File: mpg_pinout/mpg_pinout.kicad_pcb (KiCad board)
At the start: 2 copper layers, 9 parts, among them J1 Conn_02x05_Odd_Even, J2 Conn_01x02_Pin, J3 Conn_01x02_Pin, J4 Conn_01x02_Pin, J5 Conn_01x02_Pin, J6 Conn_01x02_Pin, J7 Conn_01x02_Pin, J8 Conn_01x02_Pin

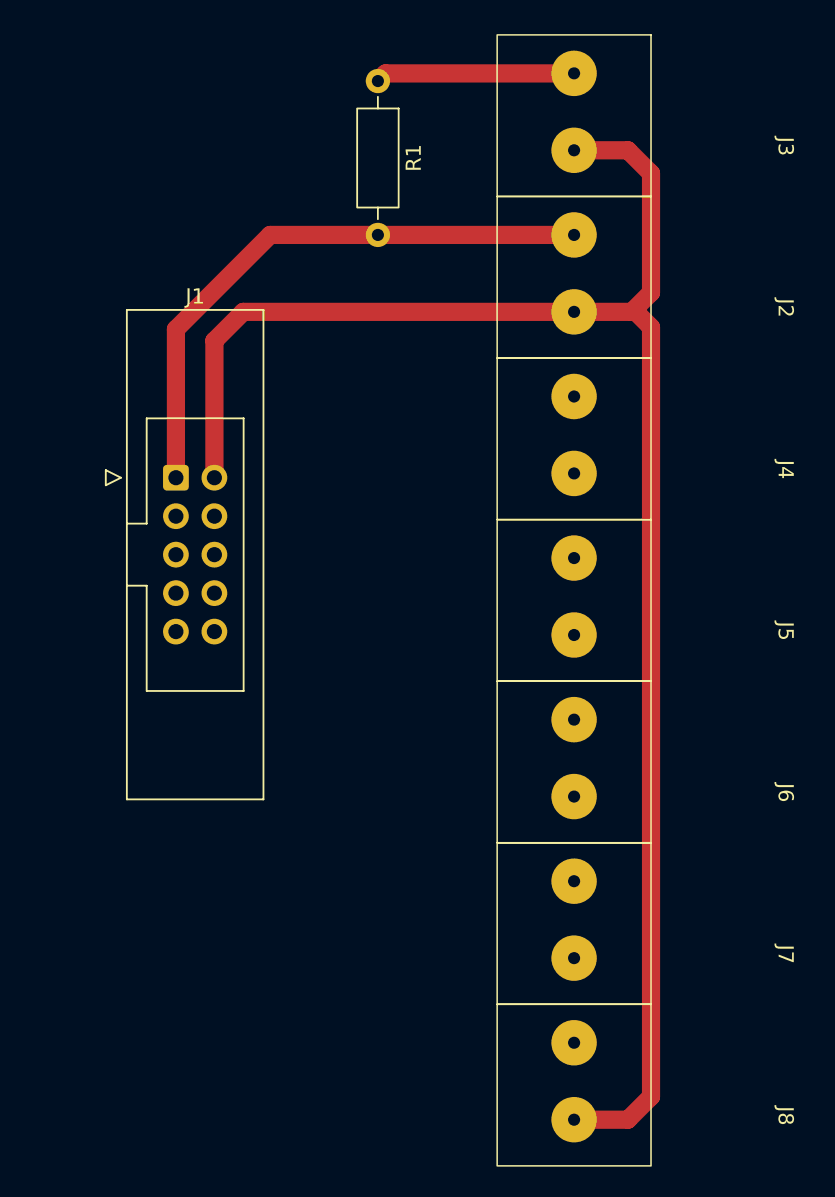
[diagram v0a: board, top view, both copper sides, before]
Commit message: third commit
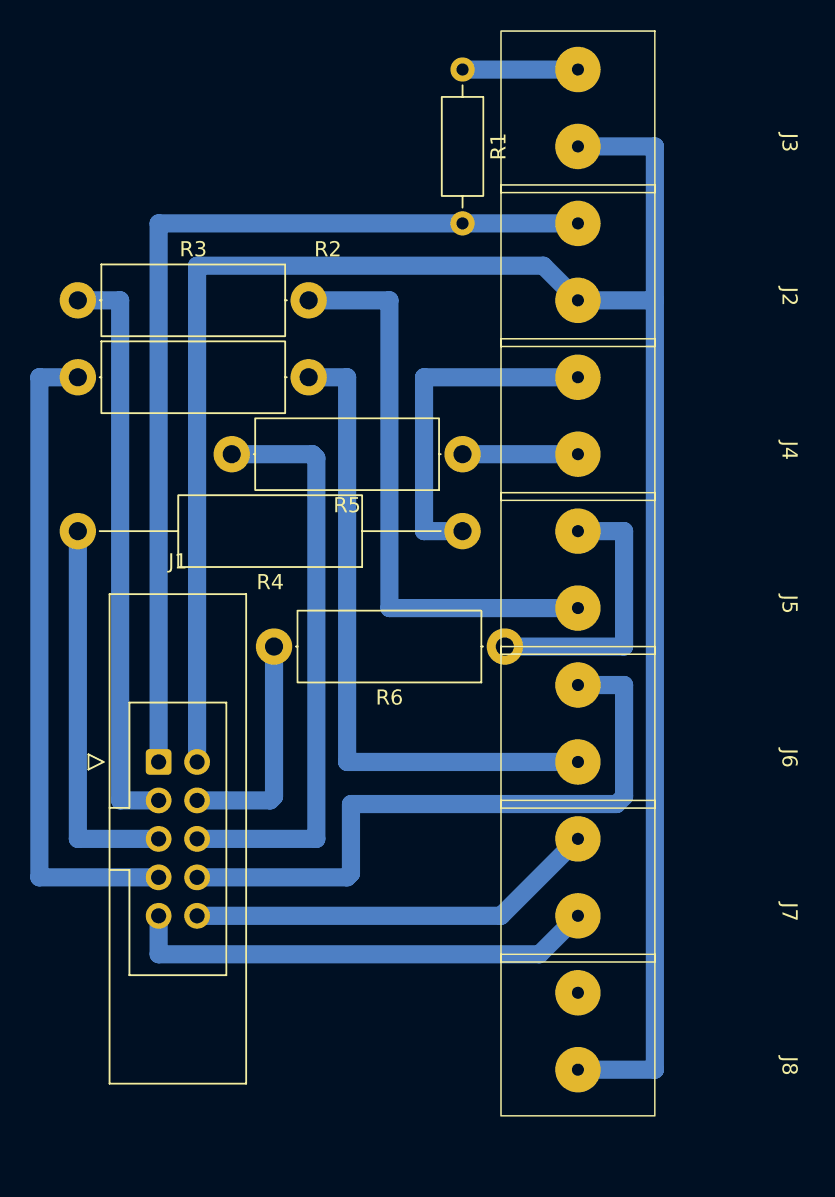
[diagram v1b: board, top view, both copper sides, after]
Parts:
- added R2: R, Resistor_THT:R_Axial_DIN0414_L11.9mm_D4.5mm_P15.24mm_Horizontal, F.Cu at (78.7, 61.0)
- added R3: R, Resistor_THT:R_Axial_DIN0414_L11.9mm_D4.5mm_P15.24mm_Horizontal, F.Cu at (78.7, 66.0)
- added R4: R, Resistor_THT:R_Axial_DIN0414_L11.9mm_D4.5mm_P25.40mm_Horizontal, F.Cu at (104.1, 76.2)
- added R5: R, Resistor_THT:R_Axial_DIN0414_L11.9mm_D4.5mm_P15.24mm_Horizontal, F.Cu at (104.1, 71.1)
- added R6: R, Resistor_THT:R_Axial_DIN0414_L11.9mm_D4.5mm_P15.24mm_Horizontal, F.Cu at (106.9, 83.8)
- moved J1 18.8 mm to (84.1, 91.4)
- moved R1 5.64 mm to (104.1, 45.7)
- moved J8 3.31 mm to (111.8, 106.7)
- moved J7 2.81 mm to (111.8, 96.5)
- moved J6 2.30 mm to (111.8, 86.4)
- moved J5 1.80 mm to (111.8, 76.2)
- moved J4 1.30 mm to (111.8, 66.0)
- moved J2 0.80 mm to (111.8, 55.9)
- moved J3 0.36 mm to (111.8, 45.7)
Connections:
- J4 pad 1: Net-(J1-Pin_5) -> Net-(J4-Pin_1)
- J4 pad 2: Net-(J1-Pin_6) -> Net-(J4-Pin_2)
- J5 pad 1: Net-(J1-Pin_4) -> Net-(J5-Pin_1)
- J5 pad 2: Net-(J1-Pin_3) -> Net-(J5-Pin_2)
- J6 pad 2: Net-(J1-Pin_7) -> Net-(J6-Pin_2)
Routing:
- net Net-(J1-Pin_8): track 0.00 -> 43.5 mm
- net Net-(J1-Pin_7): track 0.00 -> 43.4 mm
- net Net-(J6-Pin_2): track 0.00 -> 43.2 mm
- net Net-(J1-Pin_6): track 0.00 -> 38.7 mm
- net Net-(J1-Pin_3): track 0.00 -> 38.4 mm
- net Net-(J5-Pin_2): track 0.00 -> 38.1 mm
- net Net-(J1-Pin_9): track 0.00 -> 31.3 mm
- net Net-(J1-Pin_10): track 0.00 -> 27.3 mm
- net Net-(J1-Pin_5): track 0.00 -> 25.7 mm
- net Net-(J1-Pin_1): track 38.7 -> 63.2 mm
- net unconnected-(J1-Pin_2-Pad2): track 111.0 -> 135.1 mm
- net Net-(J4-Pin_1): track 0.00 -> 22.9 mm
- net Net-(J5-Pin_1): track 0.00 -> 18.5 mm
- net Net-(J1-Pin_4): track 0.00 -> 14.8 mm
- net Net-(J4-Pin_2): track 0.00 -> 7.62 mm
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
